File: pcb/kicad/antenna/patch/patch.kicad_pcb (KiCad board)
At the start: 2 copper layers, 1 part, among them P1 CONN_01X02

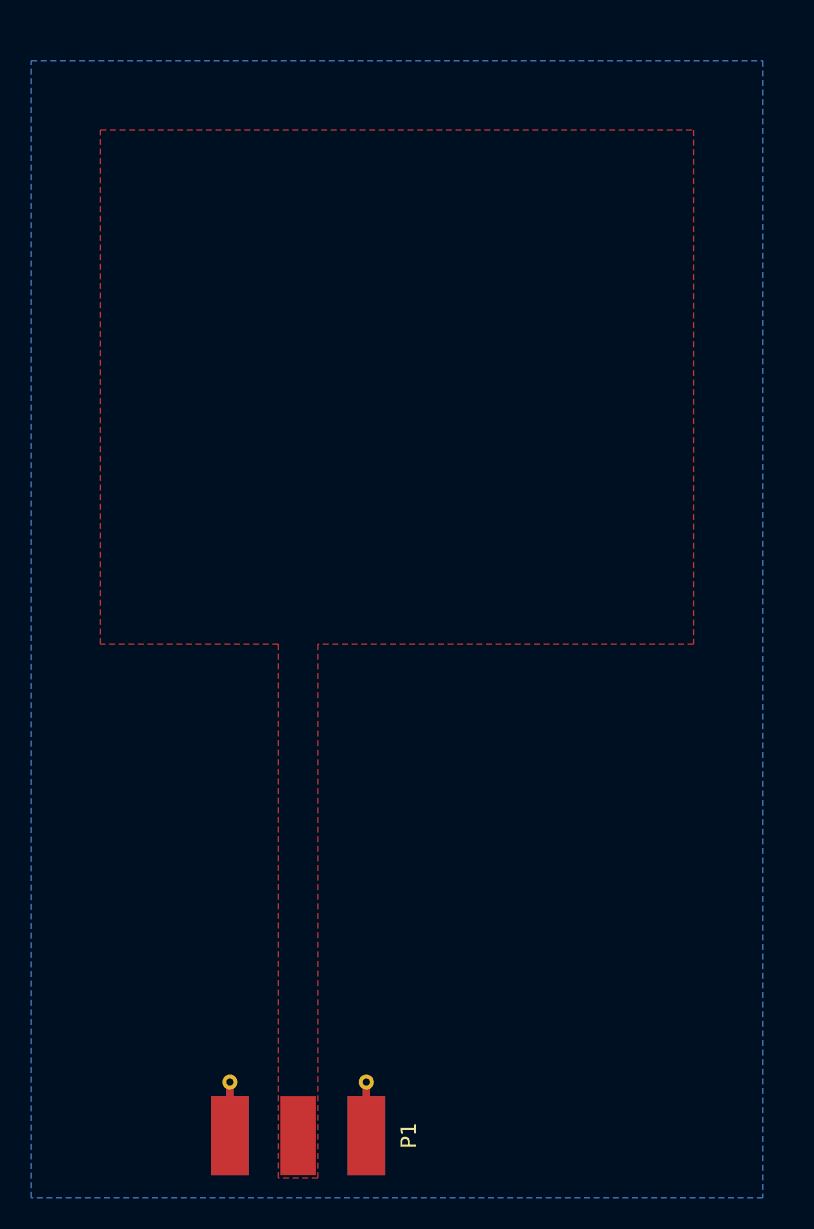
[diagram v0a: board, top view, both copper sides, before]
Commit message: Cleanup layout, files, and calculations
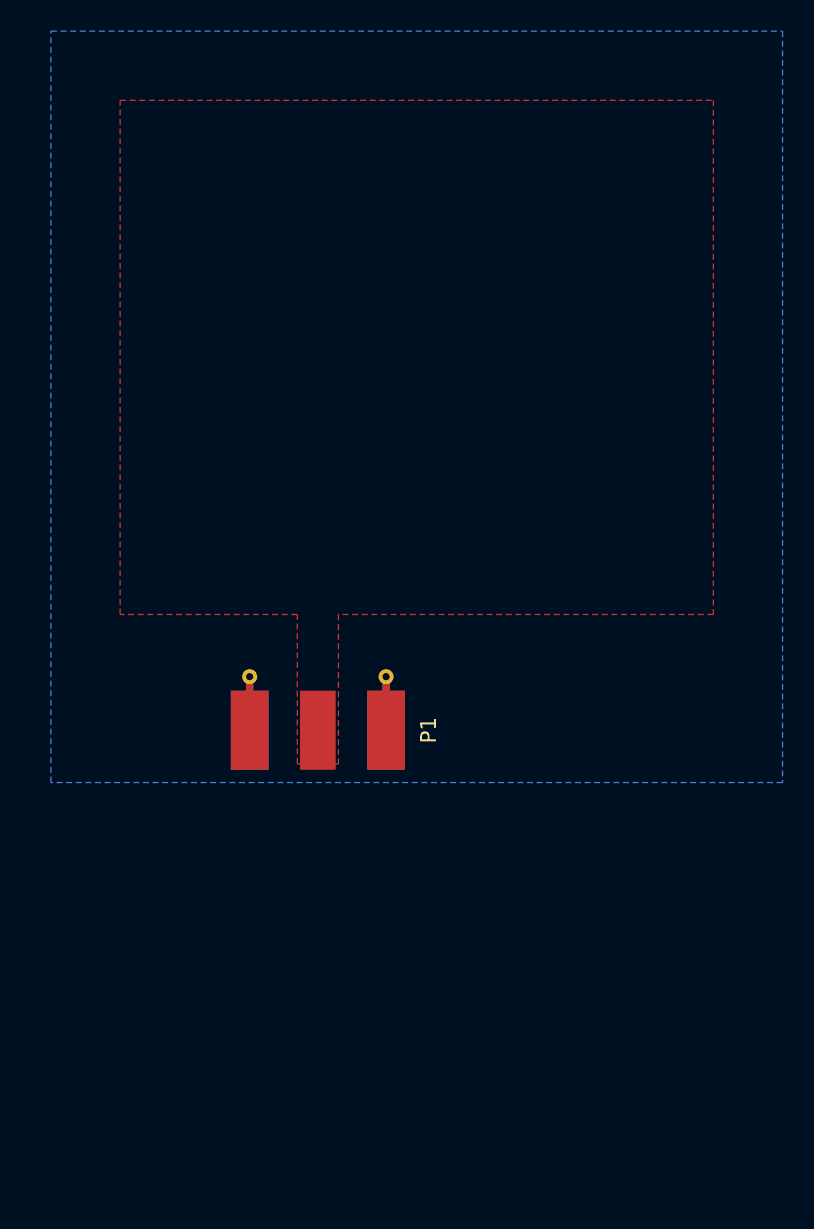
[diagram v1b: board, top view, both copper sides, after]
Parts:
- moved P1 26.1 mm to (130.2, 95.9)
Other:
- net class Default: clearance 0.2 -> 0.254; trace_width 0.25 -> 0.127; via_dia 0.6 -> 0.3556; via_drill 0.4 -> 0.254
- rule trace_clearance: 0.2 -> 0.254
- rule via_min_drill: 0.381 -> 0.254
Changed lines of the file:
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@@
     (links 9)
     (no_connects 4)
-    (area 111.76 54.61 158.750001 136.435001)
+    (area 112.929999 52.604999 272.295714 194.39)
     (thickness 1.5748)
-    (drawings 3)
+    (drawings 7)
     (tracks 0)
     (zones 0)
@@
   )
   (setup
-    (last_trace_width 0.25)
-    (user_trace_width 0.3556)
-    (user_trace_width 2.54)
-    (trace_clearance 0.2)
+    (last_trace_width 0.127)
+    (trace_clearance 0.254)
     (zone_clearance 0.508)
-    (zone_45_only no)
+    (zone_45_only yes)
     (trace_min 0.127)
     (segment_width 0.2)
     (edge_width 0.15)
-    (via_size 0.6)
-    (via_drill 0.4)
+    (via_size 0.3556)
+    (via_drill 0.254)
     (via_min_size 0.254)
-    (via_min_drill 0.381)
-    (uvia_size 0.3)
-    (uvia_drill 0.1)
+    (via_min_drill 0.254)
+    (uvia_size 0.2032)
+    (uvia_drill 0.1524)
     (uvias_allowed no)
-    (uvia_min_size 0.2286)
-    (uvia_min_drill 0.0254)
+    (uvia_min_size 0.2032)
+    (uvia_min_drill 0.1524)
     (pcb_text_width 0.3)
     (pcb_text_size 1.5 1.5)
@@
     (pad_drill 0.762)
     (pad_to_mask_clearance 0.2)
-    (aux_axis_origin 12.065 12.065)
-    (grid_origin 127.635 85.725)
+    (aux_axis_origin 113.03 100.965)
+    (grid_origin 125.73 94.615)
     (visible_elements 7FFFFFFF)
     (pcbplotparams
-      (layerselection 0x000f0_80000001)
+      (layerselection 0x030f0_80000001)
       (usegerberextensions false)
       (excludeedgelayer true)
@@
   (net 2 GND)
   (net_class Default "This is the default net class."
-    (clearance 0.2)
-    (trace_width 0.25)
-    (via_dia 0.6)
-    (via_drill 0.4)
-    (uvia_dia 0.3)
-    (uvia_drill 0.1)
+    (clearance 0.254)
+    (trace_width 0.127)
+    (via_dia 0.3556)
+    (via_drill 0.254)
+    (uvia_dia 0.2032)
+    (uvia_drill 0.1524)
     (add_net /SIG)
     (add_net GND)
   )
   (module Connectors_Molex:Molex_SMA_Jack_Edge_Mount (layer F.Cu)
-    (at 128.905 121.92 90)
+    (at 130.175 95.885 90)
     (descr "Molex SMA Jack, Edge Mount, http://www.molex.com/pdm_docs/sd/732511150_sd.pdf")
     (tags "sma edge")
@@
       (net 2 GND))
   )
+  (gr_line (start 160.02 100.965) (end 113.03 100.965) (angle 90) (layer Margin) (width 0.2))
+  (gr_line (start 160.02 52.705) (end 160.02 100.965) (angle 90) (layer Margin) (width 0.2))
+  (gr_line (start 113.03 52.705) (end 160.02 52.705) (angle 90) (layer Margin) (width 0.2))
+  (gr_line (start 113.03 100.965) (end 113.03 52.705) (angle 90) (layer Margin) (width 0.2))
   (gr_text "February 15, 2017" (at 217.17 193.04) (layer Cmts.User)
     (effects (font (size 1.5 1.5) (thickness 0.3)))
@@
     (polygon
       (pts
-        (xy 158.75 127.635) (xy 111.76 127.635) (xy 111.76 54.61) (xy 158.75 54.61)
+        (xy 113.03 52.705) (xy 160.02 52.705) (xy 160.02 100.965) (xy 113.03 100.965)
       )
     )
@@
   (zone (net 1) (net_name /SIG) (layer F.Cu) (hatch full 0.508)
     (priority 1)
-    (connect_pads yes (clearance 0.508))
+    (connect_pads (clearance 0.254))
     (min_thickness 0.254)
     (fill yes (arc_segments 16) (thermal_gap 0.508) (thermal_bridge_width 0.508))
     (polygon
       (pts
-        (xy 154.305 59.055) (xy 154.305 92.075) (xy 130.175 92.075) (xy 130.175 126.365) (xy 127.635 126.365)
-        (xy 127.635 92.075) (xy 116.205 92.075) (xy 116.205 59.055)
+        (xy 128.8542 90.17) (xy 117.475 90.17) (xy 117.475 57.15) (xy 155.575 57.15) (xy 155.575 90.17)
+        (xy 131.4958 90.17) (xy 131.4958 99.7712) (xy 128.8542 99.7712)
       )
     )
